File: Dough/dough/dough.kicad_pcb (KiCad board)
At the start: 4 copper layers, 50 x 72.5 mm, 127 parts, among them J1 BATT IN, J10 USB_ESP32, J11 Conn_01x10_Pin, J12 Conn_01x10_Pin, J2 Conn_01x05_Pin, J3 USB_RP2040, J4 servo 6, J401 SD CARD, J5 servo 1, J6 servo 2, J7 servo 3, J8 servo 4, J9 servo 5, Q1 2N7002, Q2 2N7002, Q3 AO3401A, Q4 2N7002, Q5 2N7002, SW1 2040 RST, SW2 ESP32 BOOT, SW301 2040 BOOTSEL, SW4 ESP32 RST, U1 W25Q32JVSS, U11 25SH-B-04-TS, U2 RP2040, U3 AZ1084-5.0, U4 TLV1117-33, U5 LM4040DBZ-3, U6 BMP581, U7 MMC5633NJL, U8 BMI160, U9 ESP32-S3-WROOM-1, Y1 Crystal

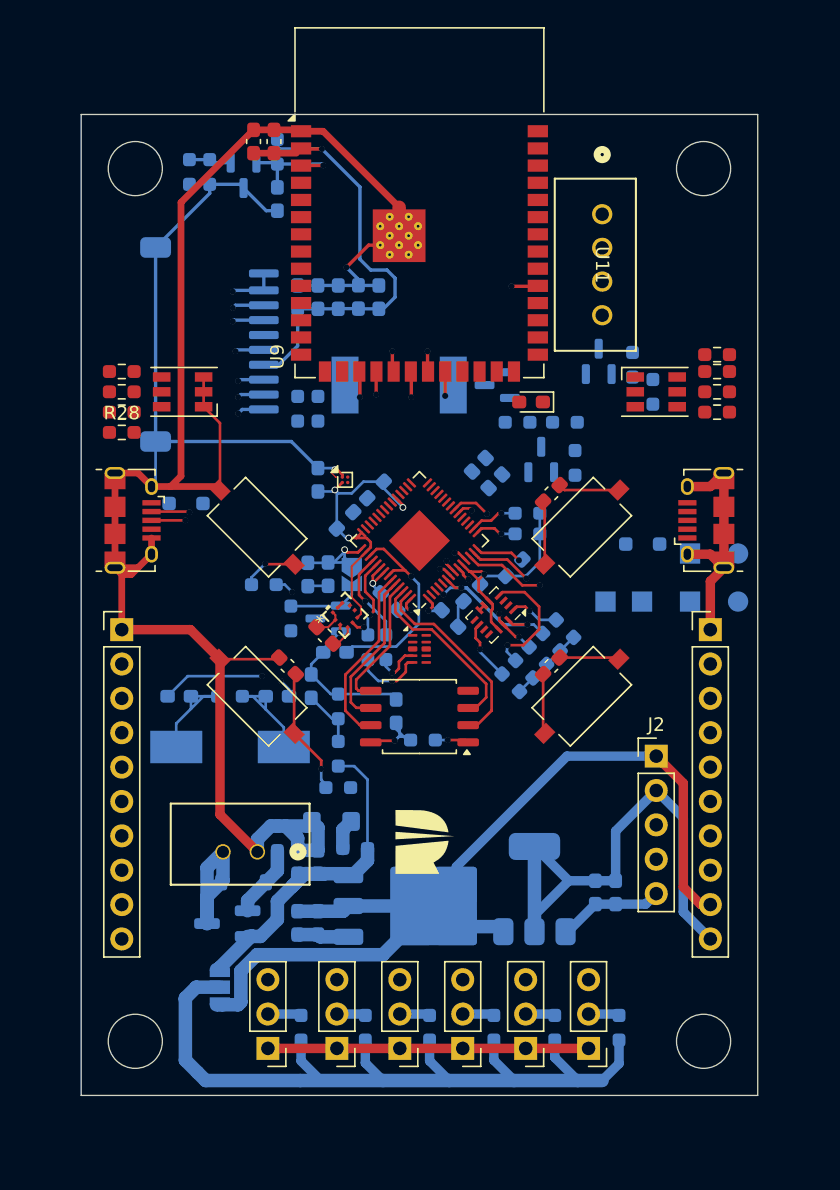
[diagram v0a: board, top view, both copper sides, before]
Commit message: pre prod 1
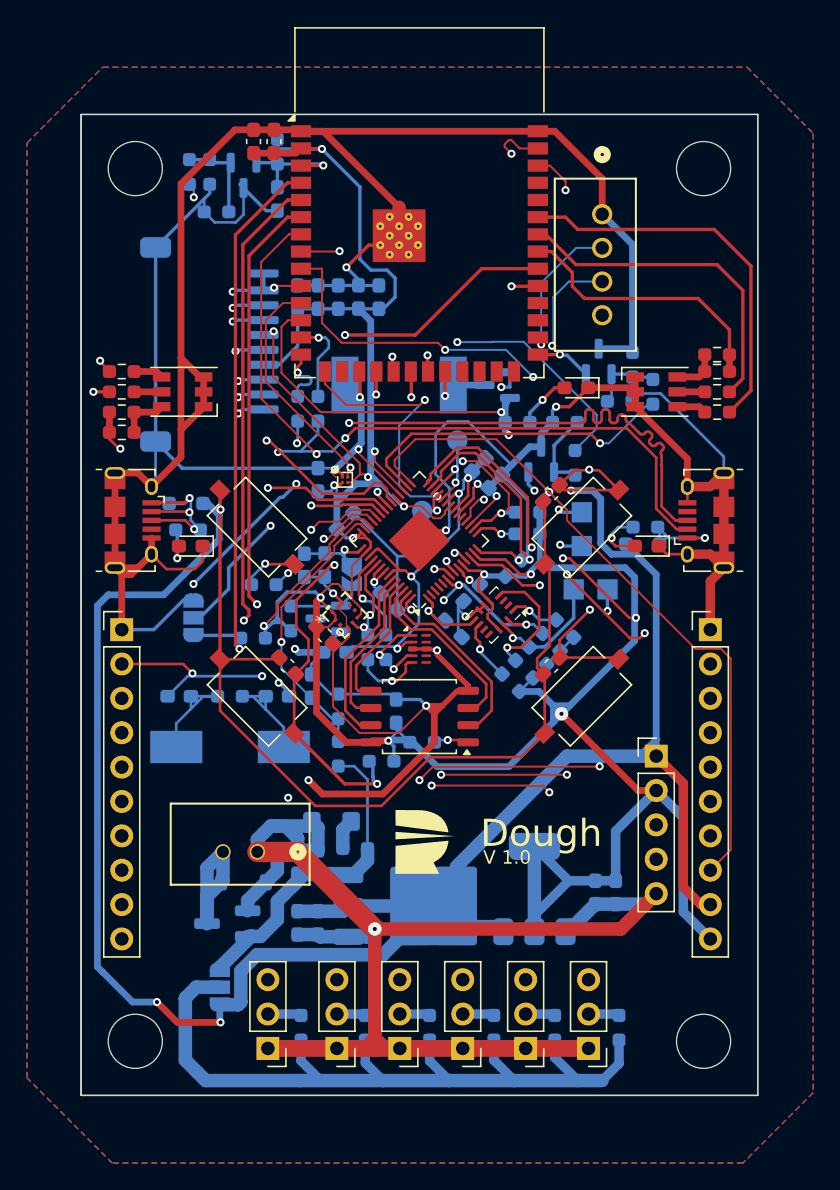
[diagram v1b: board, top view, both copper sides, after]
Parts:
- removed C29: 100n, Capacitor_SMD:C_0603_1608Metric_Pad1.08x0.95mm_HandSolder
- added D8: LED, LED_SMD:LED_0603_1608Metric_Pad1.05x0.95mm_HandSolder, F.Cu at (105.9, 67.8)
- added D9: LED, LED_SMD:LED_0603_1608Metric_Pad1.05x0.95mm_HandSolder, F.Cu at (139.6, 67.8)
- added JP3: ~, Jumper:SolderJumper-3_P1.3mm_Open_RoundedPad1.0x1.5mm, B.Cu at (106.1, 73.1)
- added R35: 10k, Resistor_SMD:R_0603_1608Metric_Pad0.98x0.95mm_HandSolder, B.Cu at (107.8, 43.1)
- added R39: 10k, Resistor_SMD:R_0603_1608Metric_Pad0.98x0.95mm_HandSolder, B.Cu at (137.6, 57.1)
- added R42: 10k, Resistor_SMD:R_0603_1608Metric_Pad0.98x0.95mm_HandSolder, B.Cu at (105.7, 66.6)
- added R43: 10k, Resistor_SMD:R_0603_1608Metric_Pad0.98x0.95mm_HandSolder, B.Cu at (139.5, 66.4)
- added R44: 10k, Resistor_SMD:R_0603_1608Metric_Pad0.98x0.95mm_HandSolder, B.Cu at (110.5, 74.6)
- moved TP2 24.3 mm to (123.0, 65.2)
- moved TP1 22.4 mm to (125.6, 60.0)
- moved TP4 10.4 mm to (134.8, 65.3)
- moved TP3 8.02 mm to (134.8, 67.8)
- moved R11 3.75 mm to (120.0, 83.7)
- moved D7 3.51 mm to (134.4, 56.1)
- moved TP6 2.70 mm to (136.7, 71.0)
- moved TP5 2.52 mm to (134.2, 71.0)
- moved C31 0.80 mm to (125.3, 73.9)
- moved C10 0.72 mm to (114.3, 69.2)
- moved C14 0.72 mm to (115.8, 69.2)
- moved R19 0.17 mm to (123.0, 82.3)
- moved R26 0.07 mm to (130.8, 65.3)
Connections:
- C11 pad 2: GND -> BUTTONS
- C25 pad 2: GND -> BUTTONS
- C402 pad 2: GND -> BUTTONS
- J4 pad 1: Net-(J4-Pin_1) -> GND
- J5 pad 1: Net-(J4-Pin_1) -> GND
- J6 pad 1: Net-(J4-Pin_1) -> GND
- J7 pad 1: Net-(J4-Pin_1) -> GND
- J8 pad 1: Net-(J4-Pin_1) -> GND
- J9 pad 1: Net-(J4-Pin_1) -> GND
- SW1 pad 1: GND -> BUTTONS
- SW2 pad 1: GND -> BUTTONS
- SW301 pad 1: GND -> BUTTONS
- SW4 pad 1: GND -> BUTTONS
- U2 pad 34: unconnected-(U2-GPIO22-Pad34) -> LED_R
- U2 pad 35: unconnected-(U2-GPIO23-Pad35) -> LED_G
- U2 pad 36: unconnected-(U2-GPIO24-Pad36) -> LED_B
- U9 pad 10: unconnected-(U9-IO17-Pad10) -> SDA1
- U9 pad 11: unconnected-(U9-IO18-Pad11) -> SCL1
- U9 pad 15: unconnected-(U9-IO3-Pad15) -> SER_3
- U9 pad 38: unconnected-(U9-IO2-Pad38) -> SER_2
- U9 pad 39: unconnected-(U9-IO1-Pad39) -> SER_1
- U9 pad 9: unconnected-(U9-IO16-Pad9) -> SER_4
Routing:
- net GND: track 232.6 -> 493.1 mm, vias 2 -> 12
- net +3V3: track 135.8 -> 269.0 mm, vias 8 -> 11
- net +5V: track 64.3 -> 153.9 mm, vias 0 -> 4
- net BUTTONS: track 0.00 -> 82.2 mm, vias 0 -> 2
- net SCL0: track 3.61 -> 77.8 mm, vias 1 -> 4
- net ADC2: track 0.00 -> 72.2 mm, vias 0 -> 3
- net USB2_D+: track 0.00 -> 70.8 mm, vias 0 -> 3
- net USB2_D-: track 0.00 -> 67.6 mm, vias 0 -> 3
- net ADC0: track 0.00 -> 66.9 mm, vias 0 -> 4
- net SDA0: track 3.20 -> 69.9 mm, vias 1 -> 3
- net ADC1: track 0.00 -> 66.0 mm, vias 0 -> 4
- net GPIO4_esp: track 0.00 -> 62.2 mm, vias 0 -> 1
- net SPI0_CS2: track 0.00 -> 60.7 mm, vias 0 -> 3
- net GPIO5_esp: track 0.00 -> 59.2 mm, vias 0 -> 1
- net GPIO6_esp: track 0.00 -> 57.1 mm, vias 0 -> 1
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- added copper zone on B.Cu, net GND
- added copper zone on F.Cu, net GND
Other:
- board text added: "Dough"
- board text added: "V 1.0"
